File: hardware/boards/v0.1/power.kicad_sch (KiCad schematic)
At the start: 65 parts, among them IC3 SP3401-02UTG, J2 USB, U20 TPS62A02DRL, U23 BQ21040DBV, U30 FUSB307BMPX, U31 TPS22929D, U32 LTC2942, U36 STM6601GU2BDM6F, U39 TPS61252DSG, U40 MIC2017YM6

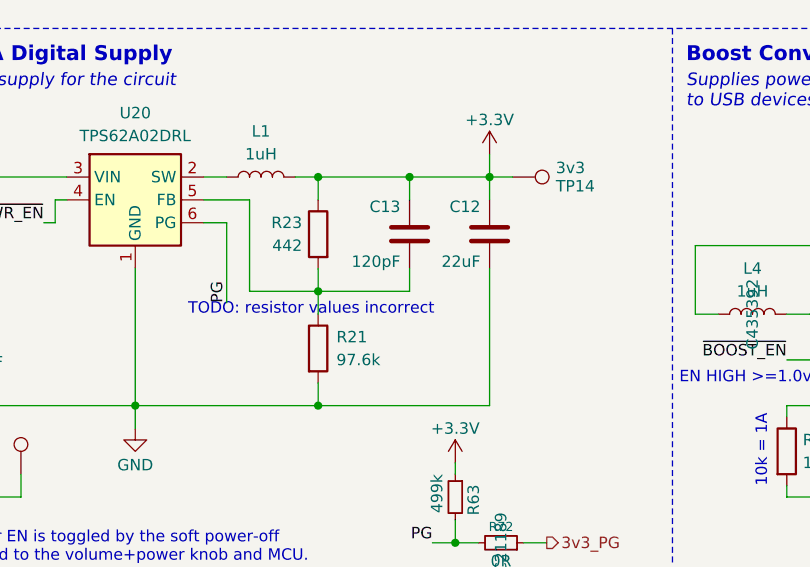
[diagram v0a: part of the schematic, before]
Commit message: feat: more BOM selection
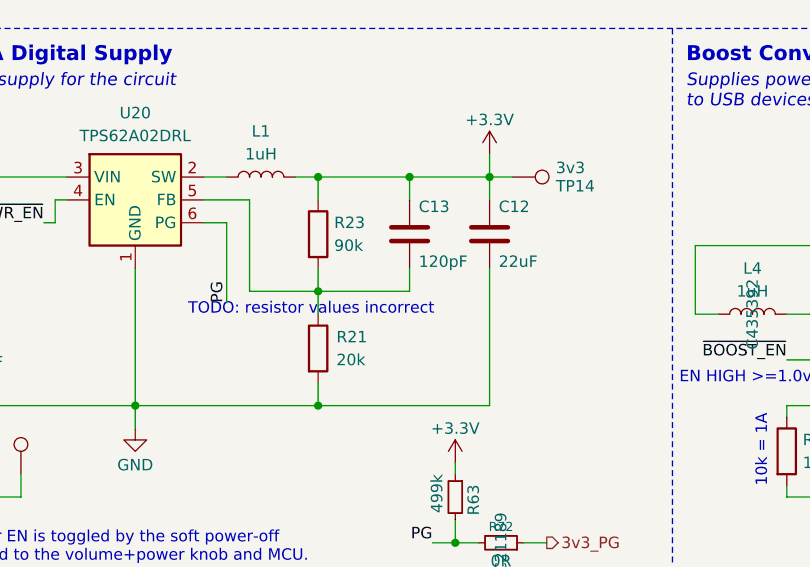
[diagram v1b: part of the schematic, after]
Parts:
- R21: value 97.6k -> 20k; footprint Resistor_SMD:R_0603_1608Metric -> Resistor_SMD:R_0402_1005Metric; JLC (none) -> C25765
- R23: value 442 -> 90k; footprint Resistor_SMD:R_0603_1608Metric -> Resistor_SMD:R_0805_2012Metric; JLC (none) -> C247028
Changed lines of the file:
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@@
 		(lib_id "Device:R")
 		(at 57.15 160.02 0)
-		(mirror y)
 		(unit 1)
 		(exclude_from_sim no)
@@
 		(dnp no)
 		(property "Reference" "R23"
-			(at 55.372 158.75 0)
+			(at 58.928 158.75 0)
 			(effects
 				(font
@@
 			)
 		)
-		(property "Value" "442"
-			(at 55.372 161.29 0)
+		(property "Value" "90k"
+			(at 58.928 161.29 0)
 			(effects
 				(font
@@
 			)
 		)
-		(property "Footprint" "Resistor_SMD:R_0603_1608Metric"
-			(at 58.928 160.02 90)
+		(property "Footprint" "Resistor_SMD:R_0805_2012Metric"
+			(at 55.372 160.02 90)
 			(effects
 				(font
@@
 			)
 		)
+		(property "JLC" "C247028"
+			(at 57.15 160.02 0)
+			(effects
+				(font
+					(size 1.27 1.27)
+				)
+				(hide yes)
+			)
+		)
 		(pin "2"
 		)
@@
 		(lib_id "Device:C")
 		(at 76.2 160.02 0)
-		(mirror y)
 		(unit 1)
 		(exclude_from_sim no)
@@
 		(dnp no)
 		(property "Reference" "C12"
-			(at 75.184 156.972 0)
+			(at 77.216 156.972 0)
 			(effects
 				(font
@@
 		)
 		(property "Value" "22uF"
-			(at 75.184 163.068 0)
+			(at 77.216 163.068 0)
 			(effects
 				(font
@@
 		)
 		(property "Footprint" "Capacitor_SMD:C_0805_2012Metric"
-			(at 75.2348 163.83 0)
+			(at 77.1652 163.83 0)
 			(effects
 				(font
@@
 			)
 		)
-		(property "Value" "97.6k"
+		(property "Value" "20k"
 			(at 59.182 173.99 0)
 			(effects
@@
 			)
 		)
-		(property "Footprint" "Resistor_SMD:R_0603_1608Metric"
+		(property "Footprint" "Resistor_SMD:R_0402_1005Metric"
 			(at 55.372 172.72 90)
 			(effects
@@
 			)
 		)
-		(property "JLC" ""
+		(property "JLC" "C25765"
 			(at 57.15 172.72 0)
 			(effects
@@
 		(lib_id "Device:C")
 		(at 67.31 160.02 0)
-		(mirror y)
 		(unit 1)
 		(exclude_from_sim no)
@@
 		(dnp no)
 		(property "Reference" "C13"
-			(at 66.294 156.972 0)
+			(at 68.326 156.972 0)
 			(effects
 				(font
@@
 		)
 		(property "Value" "120pF"
-			(at 66.294 163.068 0)
+			(at 68.326 163.068 0)
 			(effects
 				(font
@@
 		)
 		(property "Footprint" "Capacitor_SMD:C_0805_2012Metric"
-			(at 66.3448 163.83 0)
+			(at 68.2752 163.83 0)
 			(effects
 				(font
